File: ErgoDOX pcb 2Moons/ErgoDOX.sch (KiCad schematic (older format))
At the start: 64 parts, among them J1 USB, J2 3.5mm, J3 JMP, J4 JMP, SW0:10 SW0:3, SW0:11 SW0:2, SW0:12 SW0:1, SW0:7 SW0:6, SW0:8 SW0:5, SW0:9 SW0:4, SW1:10 SW1:3, SW1:11 SW1:2, SW1:12 SW1:1, SW1:13 SW1:0, SW1:9 SW1:4, SW2:10 SW2:3, SW2:11 SW2:2, SW2:12 SW2:1, SW2:13 SW2:0, SW2:7 SW2:6, SW2:8 SW2:5, SW2:9 SW2:4, SW3:10 SW3:3, SW3:11 SW3:2, SW3:12 SW3:1, SW3:13 SW3:0, SW3:8 SW3:5, SW3:9 SW3:4, SW4:10 SW4:3, SW4:11 SW4:2, SW4:12 SW4:1, SW4:13 SW4:0, SW4:7 SW4:6, SW4:8 SW4:5, SW4:9 SW4:4, SW5:10 SW5:3, SW5:11 SW5:2, SW5:12 SW5:1, SW5:13 SW5:0, SW5:7 SW5:6, SW5:8 SW5:5, SW5:9 SW5:4, U1 TEENSY2.0, U2 MCP23018

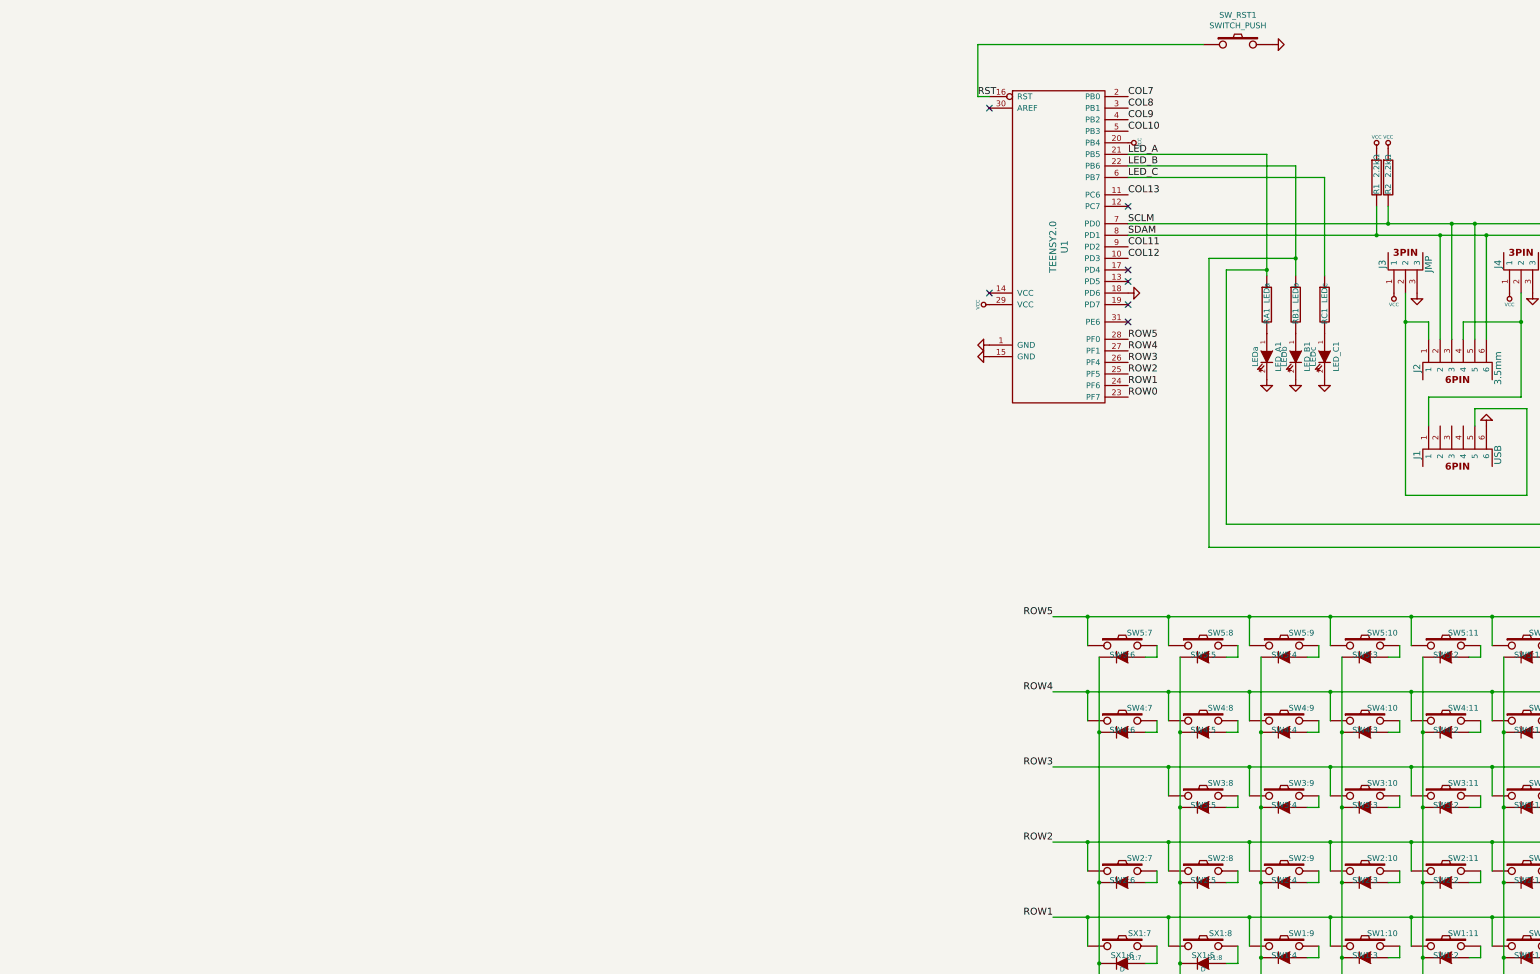
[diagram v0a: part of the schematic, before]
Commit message: New ErgoDOX PCB
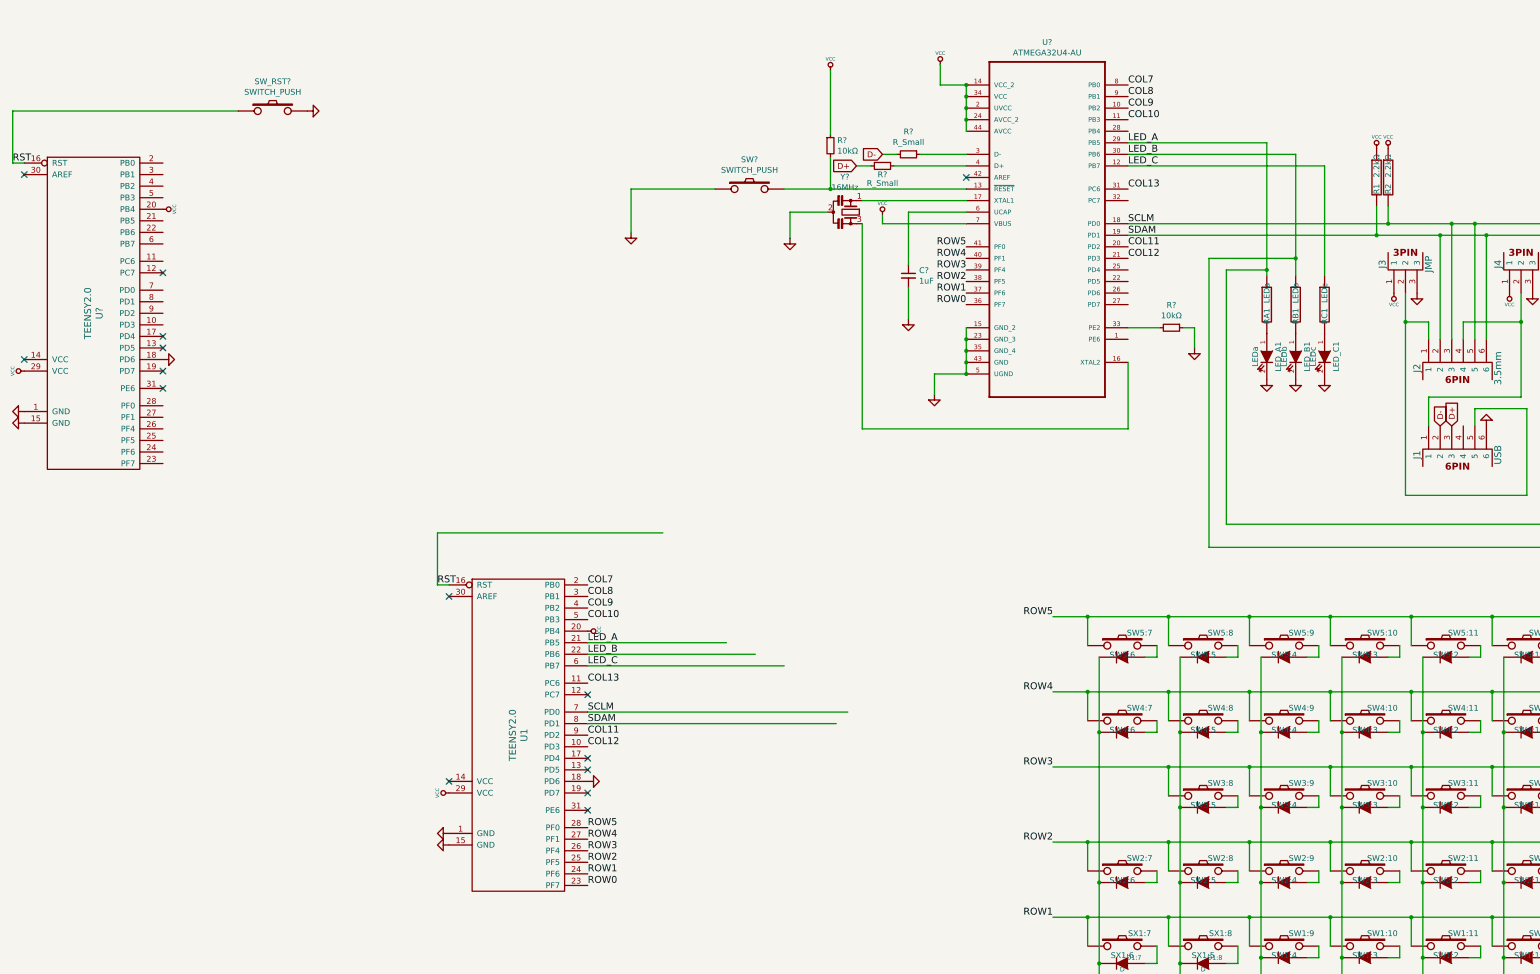
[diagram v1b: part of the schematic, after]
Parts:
- removed SW_RST1: SWITCH_PUSH, Buttons_Switches_SMD:SW_SPST_B3U-1000P, symbol component:SWITCH_PUSH
- added C?: 1uF, symbol ErgoDOX-rescue:C_Small-device
- added R? (x2): 10kΩ, symbol ErgoDOX-rescue:R_Small-device
- added R? (x2): R_Small, symbol ErgoDOX-rescue:R_Small-device
- added SW?: SWITCH_PUSH, symbol component:SWITCH_PUSH
- added SW_RST?: SWITCH_PUSH, Buttons_Switches_SMD:SW_SPST_B3U-1000P, symbol component:SWITCH_PUSH
- added U?: ATMEGA32U4-AU, QFP80P1200X1200X120-44N, symbol ErgoDOX-rescue:ATMEGA32U4-AU-ATMEGA32U4-AU
- added U?: TEENSY2.0, symbol component:TEENSY2.0
- added Y?: 16MHz, symbol ErgoDOX-rescue:Resonator_Small-device
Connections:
- net COL0: now also U?.31 (PC6)
- net COL1: now also U?.21 (PD3)
- net COL10: now also U?.11 (PB3)
- net COL11: now also U?.20 (PD2)
- net COL4: now also U?.10 (PB2)
- net COL5: now also U?.9 (PB1)
- net COL6: now also U?.8 (PB0)
- net GND: now also C?.2, R?.1, SW?.0 (GND), SW?.1, SW_RST?.0 (GND), SW_RST?.2, U?.1 (GND), U?.15 (GND), U?.15 (GND_2), U?.18 (PD6), U?.23 (GND_3), U?.35 (GND_4), U?.43 (GND), U?.5 (UGND), Y?.2
- net LED_A: now also U?.29 (PB5)
- net LED_B: now also U?.30 (PB6)
- net LED_C: now also U?.12 (PB7)
- net ROW0: now also U?.36 (PF7)
- net ROW1: now also U?.37 (PF6)
- net ROW2: now also U?.38 (PF5)
- net ROW3: now also U?.39 (PF4)
- net ROW4: now also U?.40 (PF1)
- net ROW5: now also U?.41 (PF0)
- net RST: now also SW_RST?.1, U?.16 (RST)
- net SCLM: now also U?.18 (PD0)
- net SDAM: now also U?.19 (PD1)
- net VCC: now also R?.1, U?.14 (VCC_2), U?.2 (UVCC), U?.20 (PB4), U?.24 (AVCC_2), U?.29 (VCC), U?.34 (VCC), U?.44 (AVCC), U?.7 (VBUS)
- net D-: now reaches J1.2
- net D-: now also R?.2
- net D+: now reaches J1.3
- net D+: now also R?.2
- new net: R?.2, SW?.2, U?.13 (~RESET)
- new net: U?.16 (XTAL2), Y?.3
- new net: U?.17 (XTAL1), Y?.1
- new net: R?.1, U?.3 (D-)
- new net: R?.2, U?.33 (PE2)
- new net: R?.1, U?.4 (D+)
- new net: C?.1, U?.6 (UCAP)
- no-connect marks 15 -> 23
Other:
- moved on the sheet: U1
